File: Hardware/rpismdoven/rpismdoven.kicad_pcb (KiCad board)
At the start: 2 copper layers, 2 parts

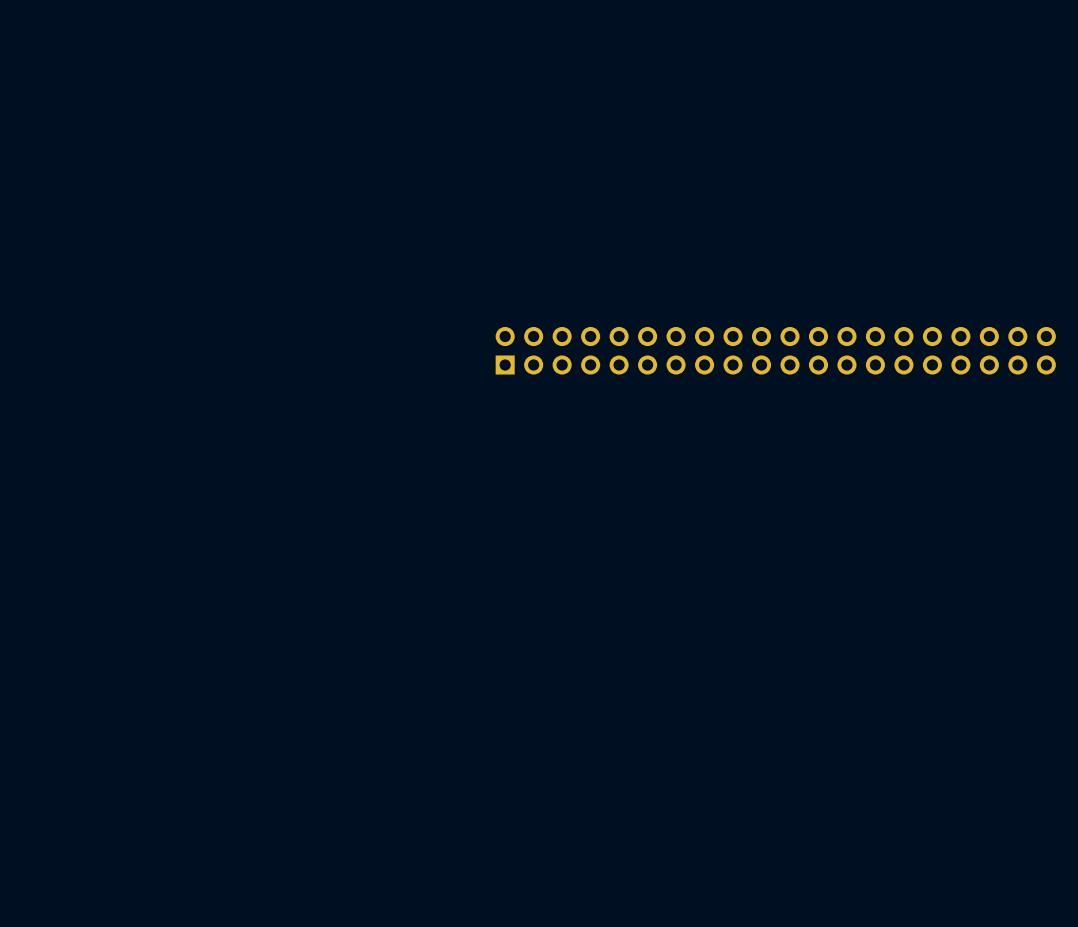
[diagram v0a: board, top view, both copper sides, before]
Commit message: bump HW
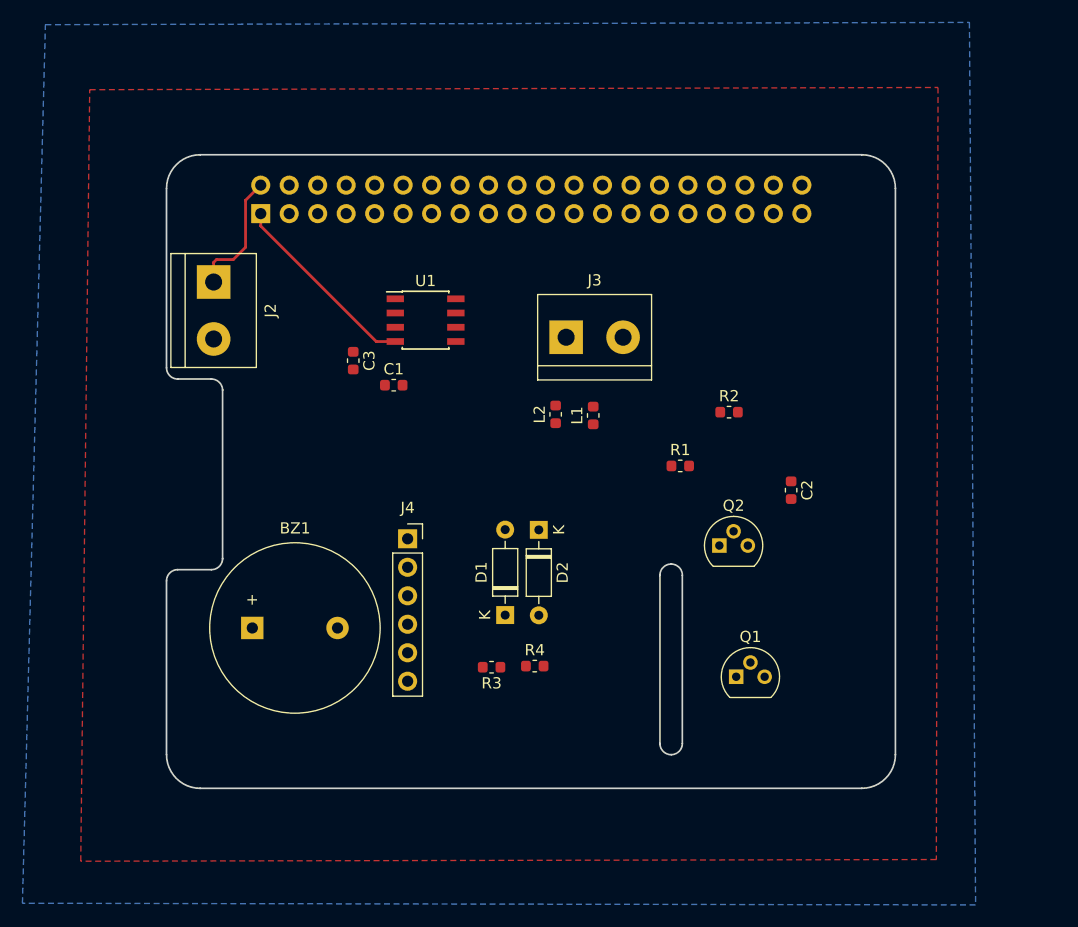
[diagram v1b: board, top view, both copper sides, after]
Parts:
- removed the REF** at (128.9, 73.7)
- added BZ1: Buzzer, Buzzer_Beeper:Buzzer_15x7.5RM7.6, F.Cu at (106.3, 97.2)
- added C1: 10nF, Capacitor_SMD:C_0603_1608Metric, F.Cu at (119.0, 75.5)
- added C2: 10uF, Capacitor_SMD:C_0603_1608Metric, F.Cu at (154.4, 84.9)
- added C3: 10uF, Capacitor_SMD:C_0603_1608Metric, F.Cu at (115.3, 73.3)
- added D1: 1N4148, Diode_THT:D_DO-35_SOD27_P7.62mm_Horizontal, F.Cu at (128.9, 96.0)
- added D2: 1N4148, Diode_THT:D_DO-35_SOD27_P7.62mm_Horizontal, F.Cu at (131.9, 88.4)
- added J1: Raspberry_Pi_2_3, Connector_PinSocket_2.54mm:PinSocket_2x20_P2.54mm_Vertical, B.Cu at (107.1, 60.2)
- added J2: Conn_01x02_Female, TerminalBlock:TerminalBlock_bornier-2_P5.08mm, F.Cu at (102.9, 66.3)
- added J3: T-PROBE, TerminalBlock:TerminalBlock_bornier-2_P5.08mm, F.Cu at (134.3, 71.2)
- added J4: MAX31855-BREAKOUT, Connector_PinSocket_2.54mm:PinSocket_1x06_P2.54mm_Vertical, F.Cu at (120.2, 89.2)
- added L1: Ferrite_Bead_Small, Inductor_SMD:L_0603_1608Metric, F.Cu at (136.8, 78.2)
- added L2: Ferrite_Bead_Small, Inductor_SMD:L_0603_1608Metric, F.Cu at (133.4, 78.1)
- added Q1: 2N2219, Package_TO_SOT_THT:TO-92, F.Cu at (149.5, 101.5)
- added Q2: 2N2219, Package_TO_SOT_THT:TO-92, F.Cu at (148.0, 89.8)
- added R1: 1k, Resistor_SMD:R_0603_1608Metric, F.Cu at (144.5, 82.7)
- added R2: 1k, Resistor_SMD:R_0603_1608Metric, F.Cu at (148.9, 77.9)
- added R3: R_Small, Resistor_SMD:R_0603_1608Metric, F.Cu at (127.7, 100.7)
- added R4: R_Small, Resistor_SMD:R_0603_1608Metric, F.Cu at (131.5, 100.5)
- added U1: MAX31855TASA, Package_SO:SOIC-8_3.9x4.9mm_P1.27mm, F.Cu at (121.8, 69.7)
- moved REF** 25.7 mm to (131.2, 83.2)
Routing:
- net +3V3: track 0.00 -> 17.4 mm
- net +5V: track 0.00 -> 11.3 mm
- added copper zone on B.Cu, net GND
- added copper zone on F.Cu, net GND
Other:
- board outline added: 65 x 56.5 mm
